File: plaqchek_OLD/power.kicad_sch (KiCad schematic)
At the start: 42 parts, among them U10 LM34601, U11 TPS7A2050PDBVR, U12 TPS54202DDC, U14 MIC5504-1.8YM5, U15 TPS62175DQC, U16 LDK320AM-R, U8 MC79M05_TO252

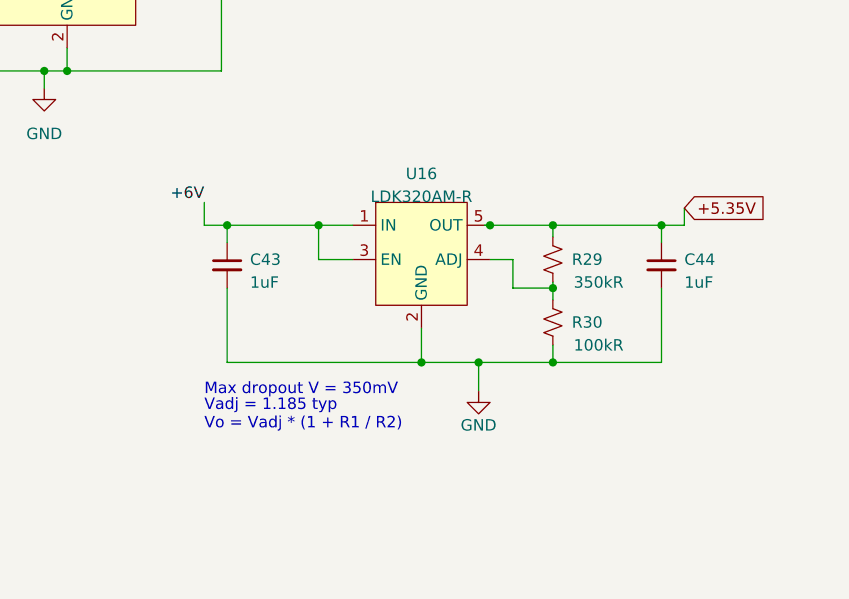
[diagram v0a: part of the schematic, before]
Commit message: finish schematic
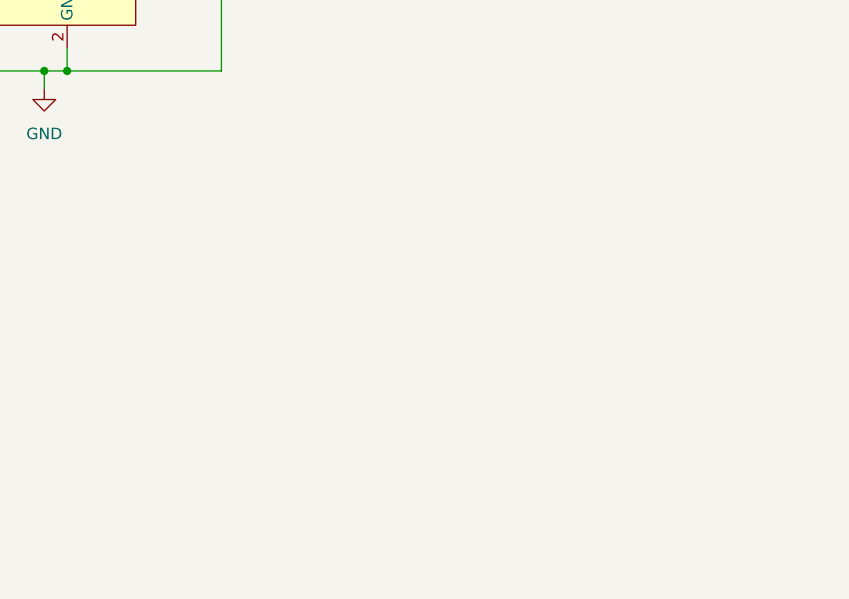
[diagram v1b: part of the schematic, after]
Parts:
- removed C43, C44: 1uF, symbol Device:C_Small
- removed R29: 350kR, symbol Device:R_Small_US
- removed R30: 100kR, symbol Device:R_Small_US
- removed U16: LDK320AM-R, symbol plaqchek_mlb:LDK320AM-R
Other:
- note removed: "Max dropout V = 350mV"
- note removed: "Vadj = 1.185 typ Vo = Vadj * (1 + R1 / R2)"
